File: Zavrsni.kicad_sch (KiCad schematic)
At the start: 38 parts, among them J1 JOYSTICK, J2 LSM6DS3, J3 ILI9341, J4 NUCLEO-H743ZI2, J5 NUCLEO-H743ZI2, J6 NUCLEO-H743ZI2, J7 NUCLEO-H743ZI2, J8 Conn_02x35_Odd_Even, J9 Conn_02x35_Odd_Even, K1 JST-2pin-SMD, Q2 BSD235C, SW1 SW_Push, SW2 SW_Push

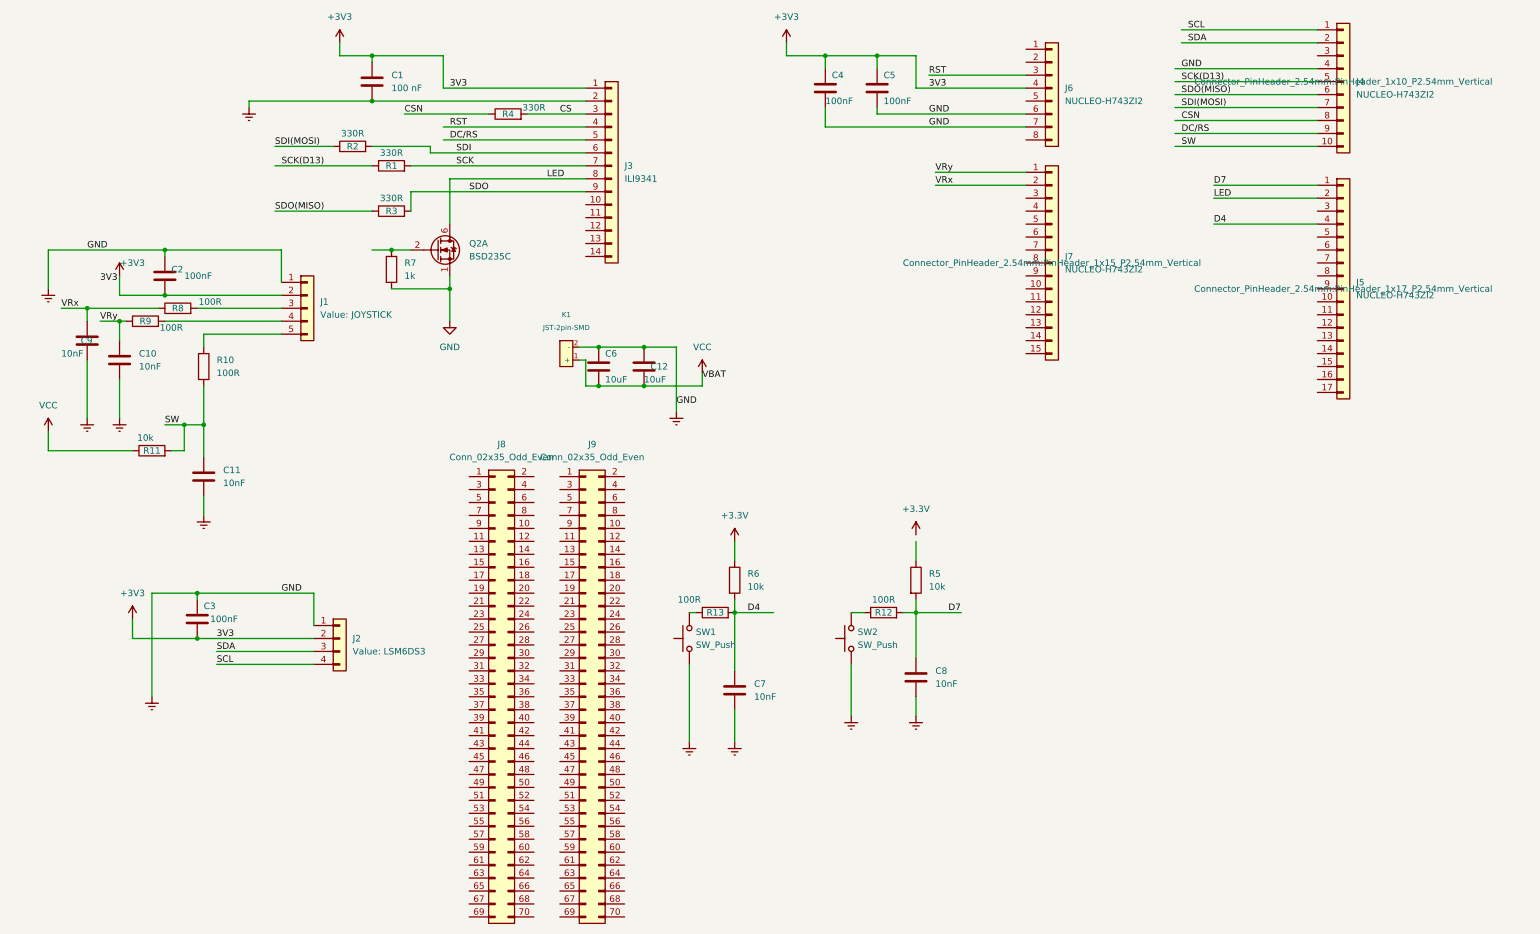
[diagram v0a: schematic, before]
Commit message: Add files via upload
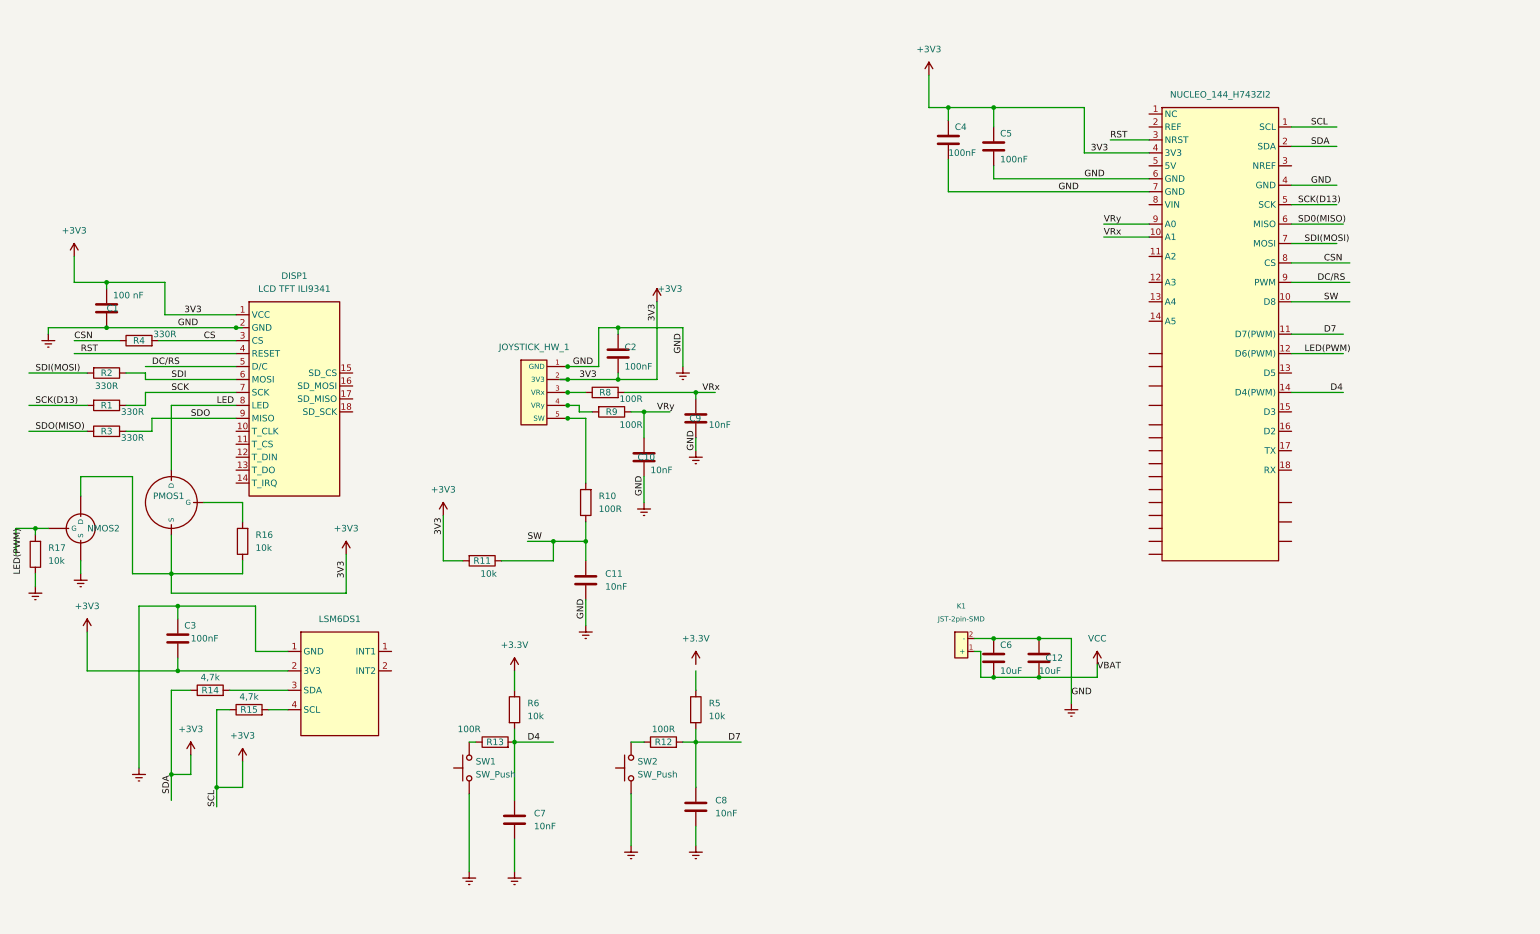
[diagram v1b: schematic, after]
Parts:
- removed J1: JOYSTICK, Connector_PinSocket_2.54mm:PinSocket_1x05_P2.54mm_Vertical, symbol Connector_Generic:Conn_01x05
- removed J2: LSM6DS3, Connector_PinSocket_2.54mm:PinSocket_1x04_P2.54mm_Vertical, symbol Connector_Generic:Conn_01x04
- removed J3: ILI9341, Connector_PinSocket_2.54mm:PinSocket_1x14_P2.54mm_Vertical, symbol Connector_Generic:Conn_01x14
- removed J4: NUCLEO-H743ZI2, Connector_PinHeader_2.54mm:PinHeader_1x10_P2.54mm_Vertical, symbol Connector_Generic:Conn_01x10
- removed J5: NUCLEO-H743ZI2, Connector_PinHeader_2.54mm:PinHeader_1x17_P2.54mm_Vertical, symbol Connector_Generic:Conn_01x17
- removed J6: NUCLEO-H743ZI2, Connector_PinHeader_2.54mm:PinHeader_1x08_P2.54mm_Vertical, symbol Connector_Generic:Conn_01x08
- removed J7: NUCLEO-H743ZI2, Connector_PinHeader_2.54mm:PinHeader_1x15_P2.54mm_Vertical, symbol Connector_Generic:Conn_01x15
- removed J8, J9: Conn_02x35_Odd_Even, Connector_PinHeader_2.54mm:PinHeader_2x35_P2.54mm_Vertical, symbol Connector_Generic:Conn_02x35_Odd_Even
- removed Q2: BSD235C, Package_TO_SOT_SMD:SOT-363_SC-70-6, symbol Transistor_FET:BSD235C
- removed R7: 1k, Resistor_SMD:R_0603_1608Metric, symbol Device:R
- added DISP1: LCD TFT ILI9341, BornaKiCad:LCD_TFT_2.4, symbol BornaLibrary:LCD_TFT_2.4
- added JOYSTICK_HW_1: ~, JOYSTICK:JOYSTICK, symbol joystick_symbol1:JOYSTICK-HW-504
- added LSM6DS1: ~, LSMDS3_akceleometar_žiroskop:LSM6DS3, symbol LSM6DS3_symbol:LSM6DS3
- added NMOS2: ~, Package_TO_SOT_SMD:SOT-23-3, symbol NMOS_symbol:NMOS
- added NUCLEO_144_H743ZI2: ~, NUCLEO_PCB:NUCLEO_PCB, symbol NUCLEO_SYMBOL:NUCLEO_144
- added PMOS1: ~, Package_TO_SOT_SMD:SOT-23-3, symbol PMOS_symbol:PMOS
- added R14, R15: 4,7k, Resistor_SMD:R_0603_1608Metric, symbol Device:R
- added R16, R17: 10k, symbol Device:R
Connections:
- net +3V3: now also R11.2, DISP1.1 (VCC), JOYSTICK_HW_1.2 (3V3), LSM6DS1.2 (INT2), NMOS2. (S), NUCLEO_144_H743ZI2.1 (SCL), NUCLEO_144_H743ZI2.2 (SDA), NUCLEO_144_H743ZI2.4 (GND), PMOS1. (S), R14.1, R15.1, R16.1
- net CS: now also DISP1.3 (CS)
- net CSN: now also NUCLEO_144_H743ZI2.8 (VIN)
- net D4: now also NUCLEO_144_H743ZI2.14 (D4(PWM))
- net D7: now also NUCLEO_144_H743ZI2.11 (D7(PWM))
- net DC/RS: now also DISP1.5 (D/C), NUCLEO_144_H743ZI2.9 (PWM)
- net Earth: now also DISP1.2 (GND), JOYSTICK_HW_1.1 (GND), LSM6DS1.1 (INT1), NMOS2. (S), NUCLEO_144_H743ZI2.4 (GND), NUCLEO_144_H743ZI2.6 (MISO), NUCLEO_144_H743ZI2.7 (MOSI), R17.1
- net LED: now also DISP1.8 (LED), PMOS1. (S)
- net RST: now also DISP1.4 (RESET), NUCLEO_144_H743ZI2.3 (NRST)
- net SCK: now also R1.1, DISP1.7 (SCK); no longer R1.2
- net SCK(D13): now also R1.2, NUCLEO_144_H743ZI2.5 (SCK); no longer R1.1
- net SDI: now also R2.1, DISP1.6 (MOSI); no longer R2.2
- net SDI(MOSI): now also R2.2, NUCLEO_144_H743ZI2.7 (MOSI); no longer R2.1
- net SDO: now also DISP1.9 (MISO)
- net SW: now also R10.1, R11.1, NUCLEO_144_H743ZI2.10 (D8); no longer R10.2, R11.2
- net VCC: no longer R11.1
- net VRx: now also R8.2, NUCLEO_144_H743ZI2.10 (D8); no longer R8.1
- net VRy: now also NUCLEO_144_H743ZI2.9 (PWM)
- net at R9.2: now also JOYSTICK_HW_1.4 (VRy)
- new net: LSM6DS1.4 (SCL), R15.2
- new net: PMOS1. (S), R16.2
- new net: LSM6DS1.3 (SDA), R14.2
- new net: JOYSTICK_HW_1.3 (VRx), R8.1
- new net: JOYSTICK_HW_1.5 (SW), R10.2
- new net LED(PWM): NMOS2. (S), NUCLEO_144_H743ZI2.12 (D6(PWM)), R17.2
- new net SD0(MISO): NUCLEO_144_H743ZI2.6 (MISO)
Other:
- moved on the sheet: C1, C10, C11, C12, C2, C3, C4, C5, C6, C7, C8, C9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
